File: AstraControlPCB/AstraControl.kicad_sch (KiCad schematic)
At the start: 0 parts

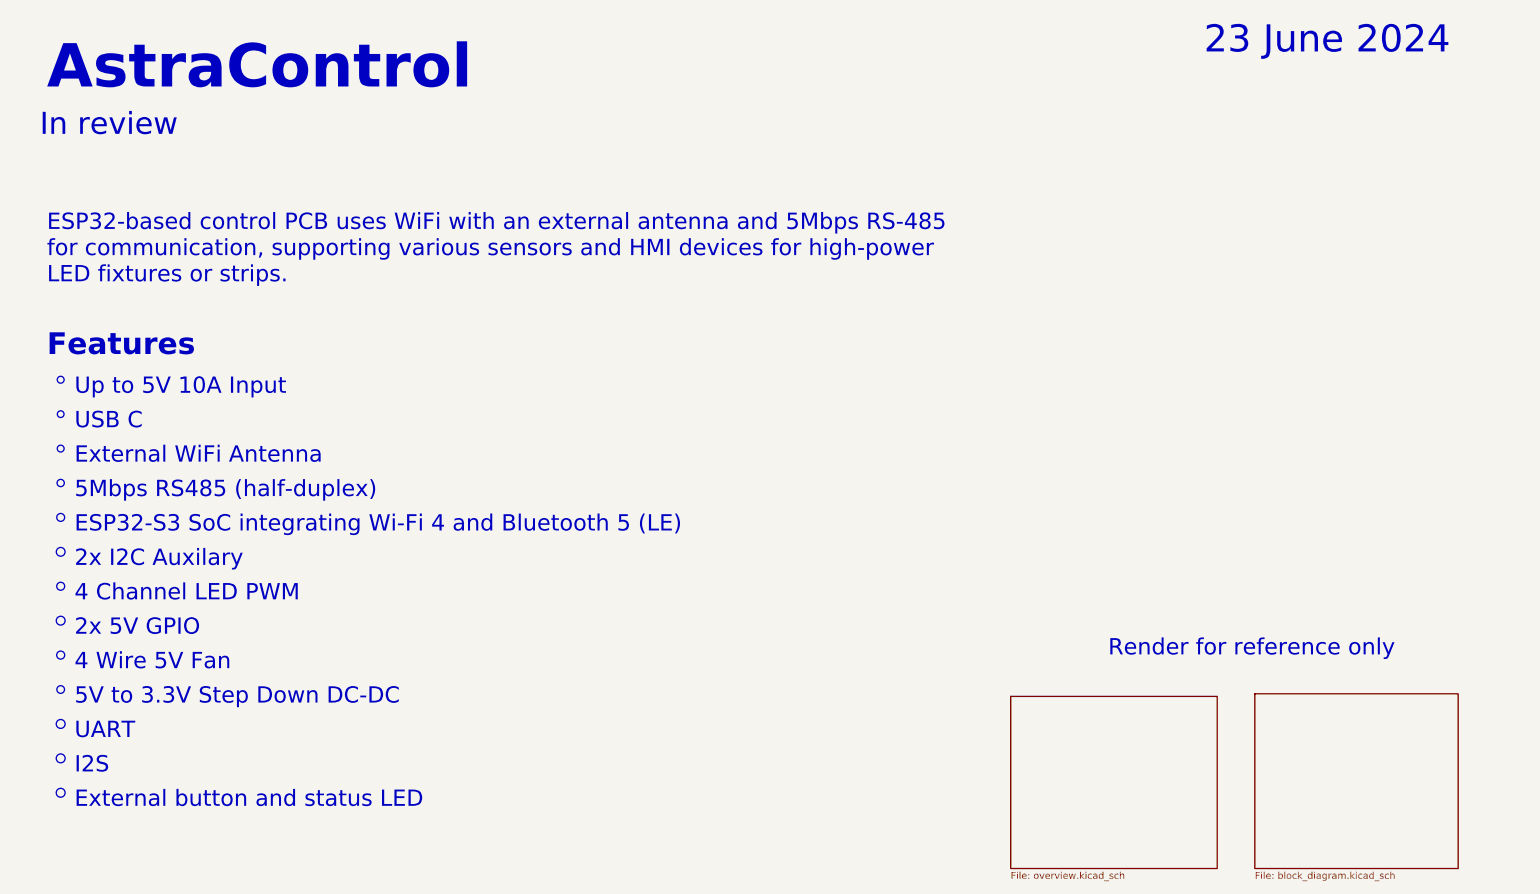
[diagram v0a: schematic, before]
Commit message: workflow
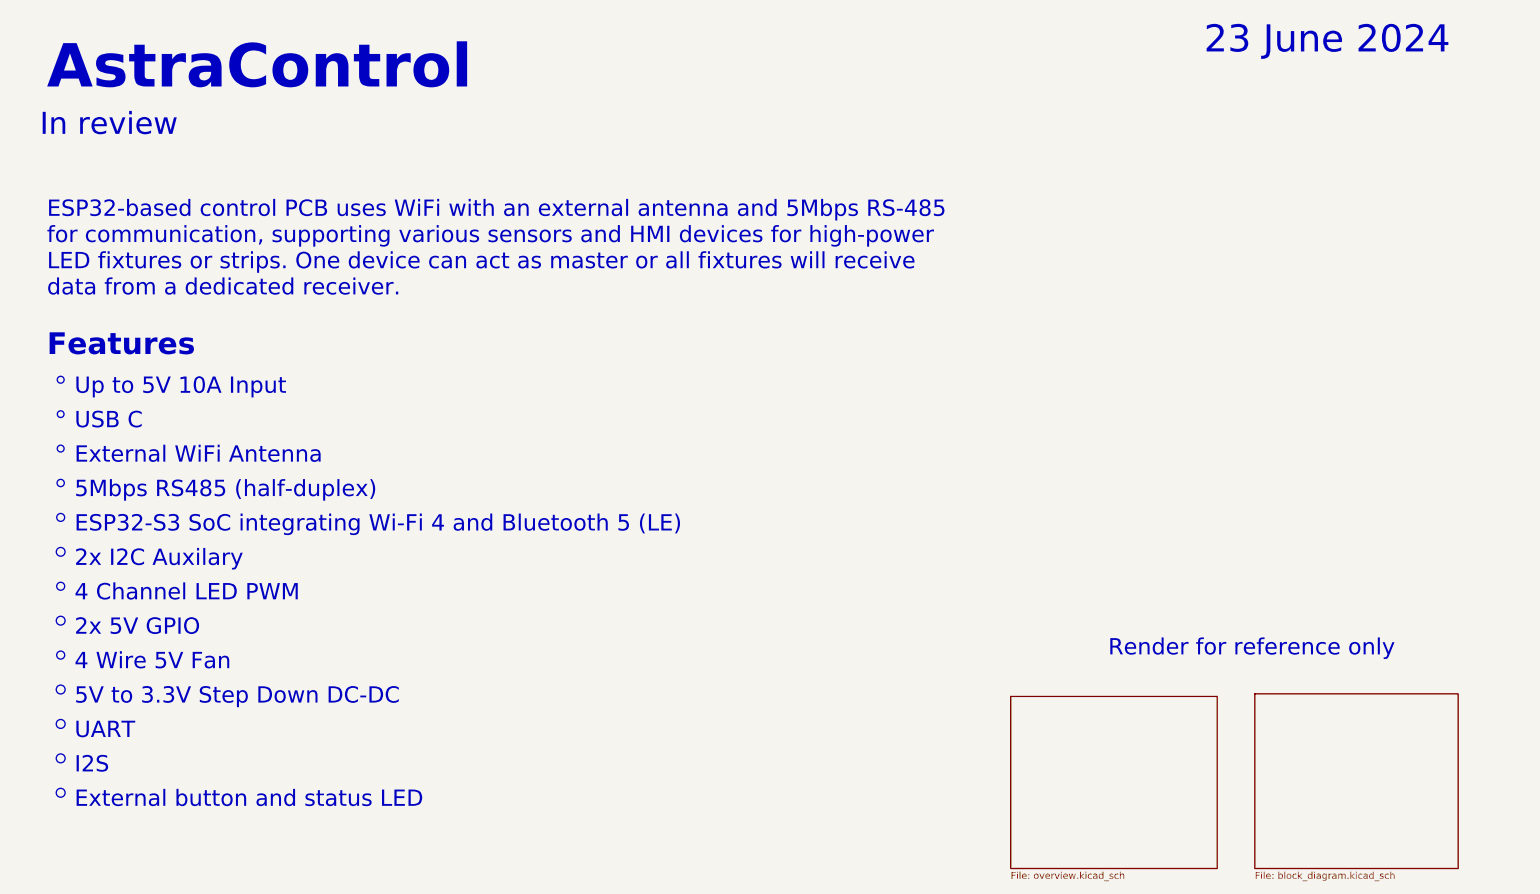
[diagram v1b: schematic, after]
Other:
- note added: "ESP32-based control PCB uses WiFi with an external antenna and 5Mbps RS-485 for communication, supporting various sensors and HMI devices for high-power LED fixtures or strips. One device can act as master or all fixtures will receive data from a dedicated receiver."
- note removed: "ESP32-based control PCB uses WiFi with an external antenna and 5Mbps RS-485 for communication, supporting various sensors and HMI devices for high-power LED fixtures or strips."
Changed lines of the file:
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@@
 		(fill
 			(type color)
-			(color 255 255 255 1)
+			(color 0 0 0 0)
 		)
 	)
 	(circle
-		(center 21.59 93.98)
-		(radius 0.6174)
+		(center 21.59 144.78)
+		(radius 0.82)
 		(stroke
 			(width -0.0001)
@@
 		(fill
 			(type color)
-			(color 255 255 255 1)
+			(color 0 0 0 0)
 		)
 	)
 	(circle
-		(center 21.59 144.78)
-		(radius 0.7071)
+		(center 21.59 93.98)
+		(radius 0.6174)
 		(stroke
 			(width -0.0001)
@@
 		(fill
 			(type color)
-			(color 255 255 255 1)
+			(color 0 0 0 0)
 		)
 	)
@@
 		(fill
 			(type color)
-			(color 255 255 255 1)
+			(color 0 0 0 0)
 		)
 	)
 	(circle
-		(center 21.59 106.68)
-		(radius 0.6696)
+		(center 21.59 151.13)
+		(radius 0.82)
 		(stroke
 			(width -0.0001)
@@
 		(fill
 			(type color)
-			(color 255 255 255 1)
+			(color 0 0 0 0)
 		)
 	)
 	(circle
-		(center 21.59 113.03)
-		(radius 0.73)
+		(center 21.59 106.68)
+		(radius 0.6696)
 		(stroke
 			(width -0.0001)
@@
 		(fill
 			(type color)
-			(color 255 255 255 1)
+			(color 0 0 0 0)
 		)
 	)
 	(circle
-		(center 21.59 100.33)
-		(radius 0.6306)
+		(center 21.59 113.03)
+		(radius 0.73)
 		(stroke
 			(width -0.0001)
@@
 		(fill
 			(type color)
-			(color 255 255 255 1)
+			(color 0 0 0 0)
 		)
 	)
 	(circle
-		(center 21.59 157.48)
-		(radius 0.82)
+		(center 21.59 100.33)
+		(radius 0.6306)
 		(stroke
 			(width -0.0001)
@@
 		(fill
 			(type color)
-			(color 255 255 255 1)
+			(color 0 0 0 0)
 		)
 	)
@@
 		(fill
 			(type color)
-			(color 255 255 255 1)
+			(color 0 0 0 0)
 		)
 	)
 	(circle
-		(center 21.59 151.13)
+		(center 21.59 157.48)
 		(radius 0.82)
 		(stroke
@@
 		(fill
 			(type color)
-			(color 255 255 255 1)
+			(color 0 0 0 0)
 		)
 	)
@@
 		(fill
 			(type color)
-			(color 255 255 255 1)
+			(color 0 0 0 0)
 		)
 	)
@@
 		(fill
 			(type color)
-			(color 255 255 255 1)
+			(color 0 0 0 0)
 		)
 	)
@@
 		(fill
 			(type color)
-			(color 255 255 255 1)
+			(color 0 0 0 0)
 		)
 	)
@@
 				(face "ING Me")
 				(size 3 3)
-				(color 255 255 255 1)
 			)
 			(justify left)
@@
 		)
 	)
-	(text "ESP32-based control PCB uses WiFi with an external antenna and 5Mbps RS-485\nfor communication, supporting various sensors and HMI devices for high-power \nLED fixtures or strips."
+	(text "ESP32-based control PCB uses WiFi with an external antenna and 5Mbps RS-485\nfor communication, supporting various sensors and HMI devices for high-power \nLED fixtures or strips. One device can act as master or all fixtures will receive \ndata from a dedicated receiver."
 		(exclude_from_sim no)
 		(at 19.05 63.5 0)
@@
 				(face "ING Me")
 				(size 3 3)
-				(color 255 255 255 1)
 			)
 			(justify left)
@@
 				(face "ING Me")
 				(size 3 3)
-				(color 255 255 255 1)
 			)
 			(justify left)
@@
 				(face "ING Me")
 				(size 3 3)
-				(color 255 255 255 1)
 			)
 			(justify left)
@@
 				(face "ING Me")
 				(size 3 3)
-				(color 255 255 255 1)
 			)
 			(justify left)
